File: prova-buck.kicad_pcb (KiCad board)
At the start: 4 copper layers, 42 x 18 mm, 21 parts, among them J1 Screw_Terminal_01x02, J2 Screw_Terminal_01x02, U1 MPQ9841GL

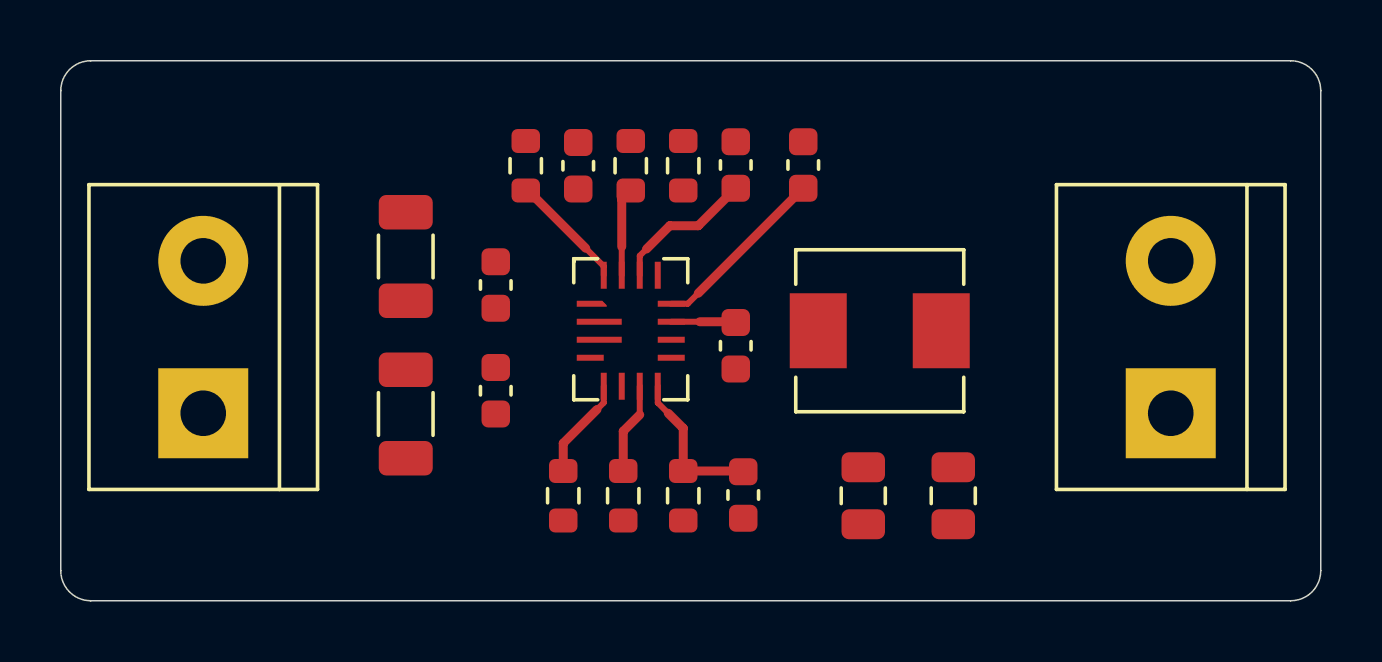
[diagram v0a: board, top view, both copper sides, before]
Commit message: "second commit"
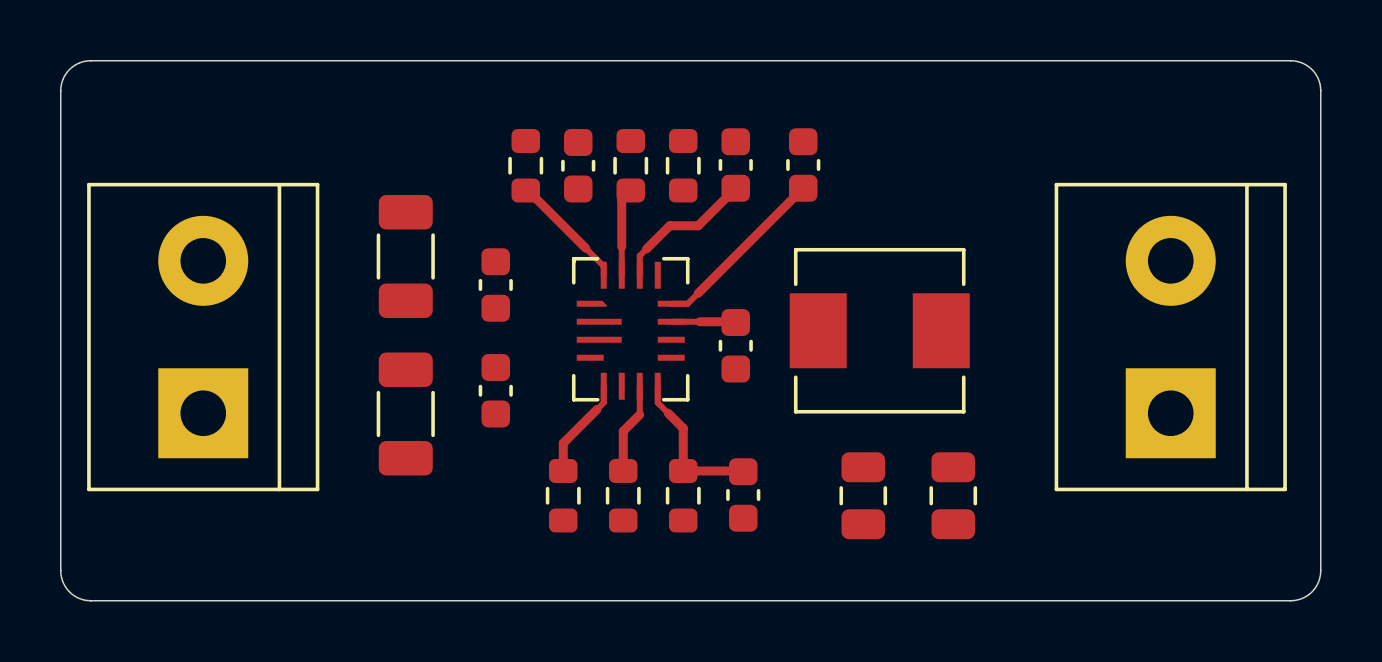
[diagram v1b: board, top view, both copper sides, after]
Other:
- net class Default removed
